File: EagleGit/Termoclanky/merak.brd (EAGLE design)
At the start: 71.1 x 39 mm, 14 parts

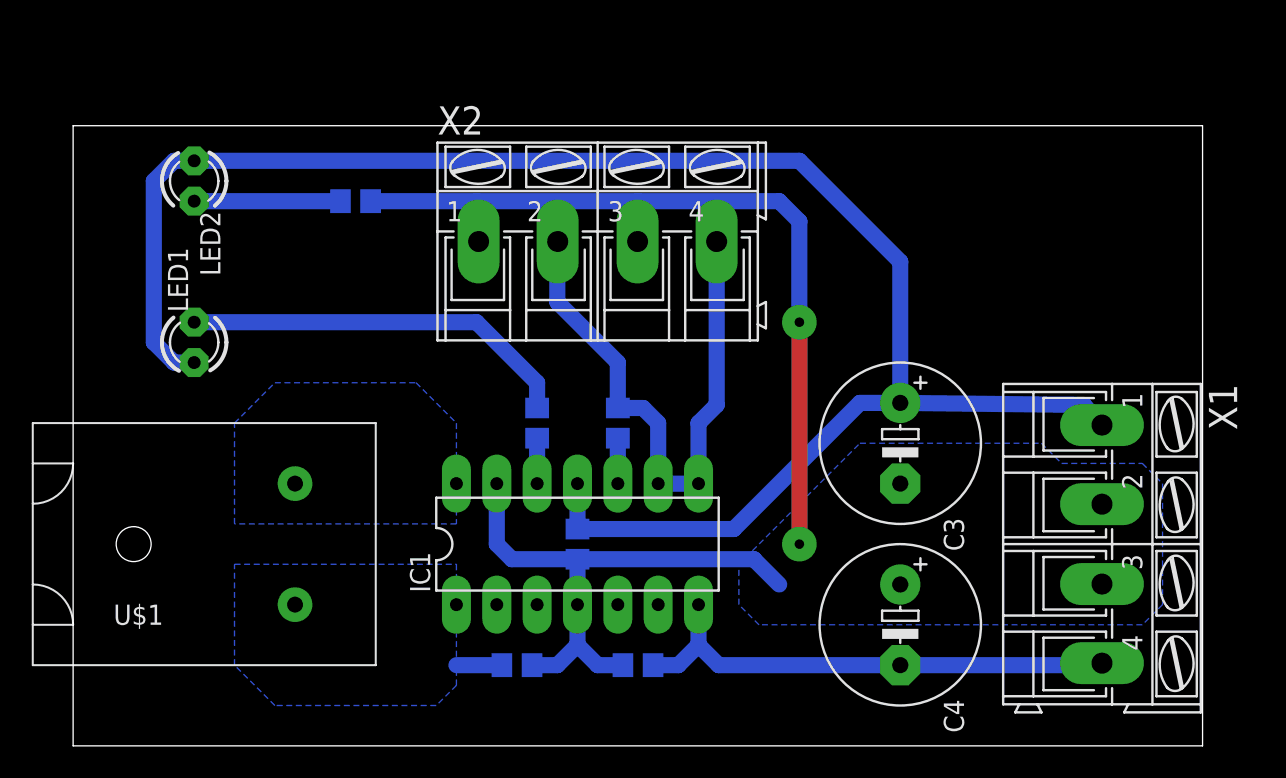
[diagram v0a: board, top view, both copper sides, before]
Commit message: Termoclanky + manuskript: - priprava do rtf
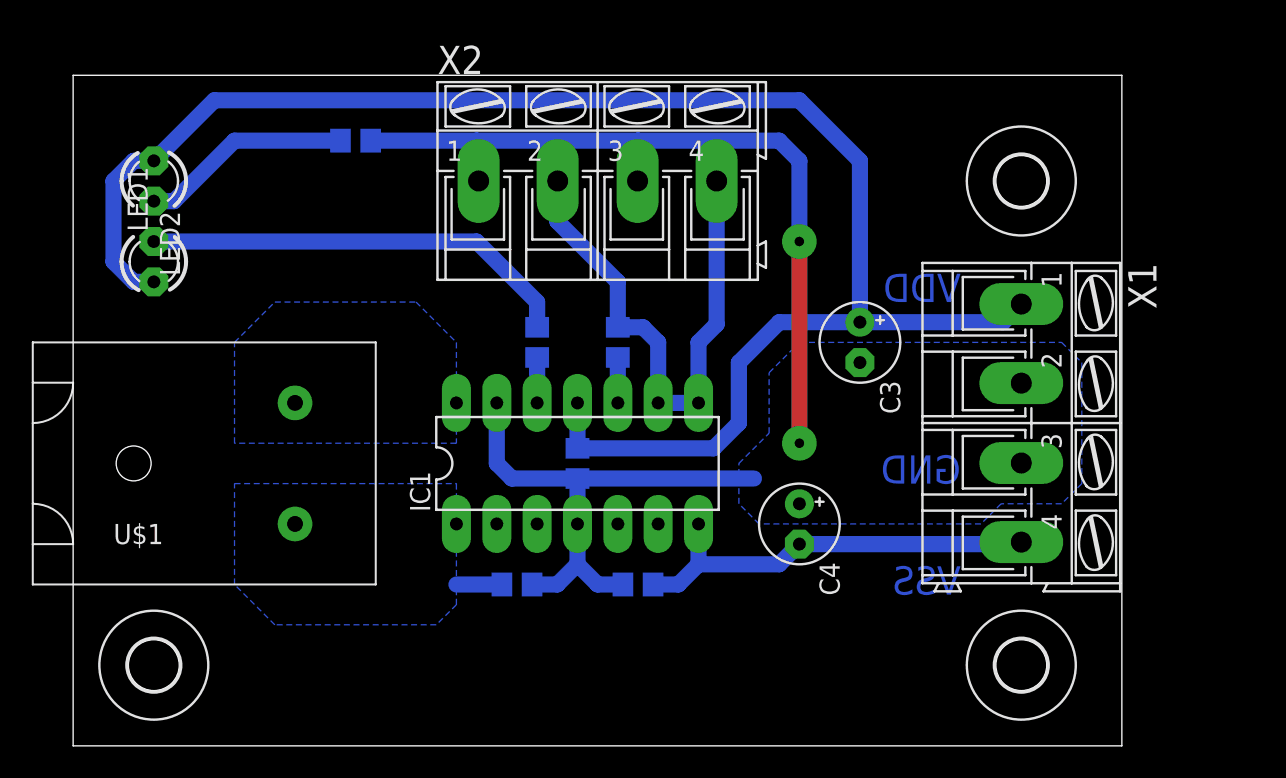
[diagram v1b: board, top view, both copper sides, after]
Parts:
- added U$2, U$3, U$4: (no value), holes:3,2
- C1, C2: value (none) -> 10n
- C3, C4: value (none) -> 10u; device rcl:E5-10,5 -> rcl:E2,5-5
- R1: value (none) -> 2k2
- moved X1 9.16 mm to (59.7, 20.3)
- moved C4 8.98 mm to (45.7, 14.0)
- moved C3 6.84 mm to (49.5, 25.4)
- moved LED1 5.68 mm to (5.08, 30.5)
- moved C1 5.08 mm to (31.8, 17.8)
- moved IC1 5.08 mm to (31.8, 17.8)
- moved U$1 5.08 mm to (11.4, 17.8)
- moved C2 5.08 mm to (35.6, 10.2)
- moved R1 5.08 mm to (27.9, 10.2)
- moved C5 5.08 mm to (34.3, 25.4)
- moved R2 5.08 mm to (29.2, 25.4)
- moved R3 3.81 mm to (17.8, 38.1)
- moved X2 3.81 mm to (33.0, 35.6)
- moved LED2 2.54 mm to (5.08, 35.6)
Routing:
- net VDD: track 112.0 -> 105.8 mm
- net VSS: track 31.9 -> 26.8 mm
- net GND: track 87.8 -> 83.0 mm
- net N$6: track 9.21 -> 13.3 mm
- net N$1: track 37.1 -> 34.5 mm
- net N$5: track 24.8 -> 27.3 mm
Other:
- board size 71.1 x 39 mm -> 66 x 42.2 mm
- board text added: "GND"
- board text added: "VDD"
- board text added: "VSS"

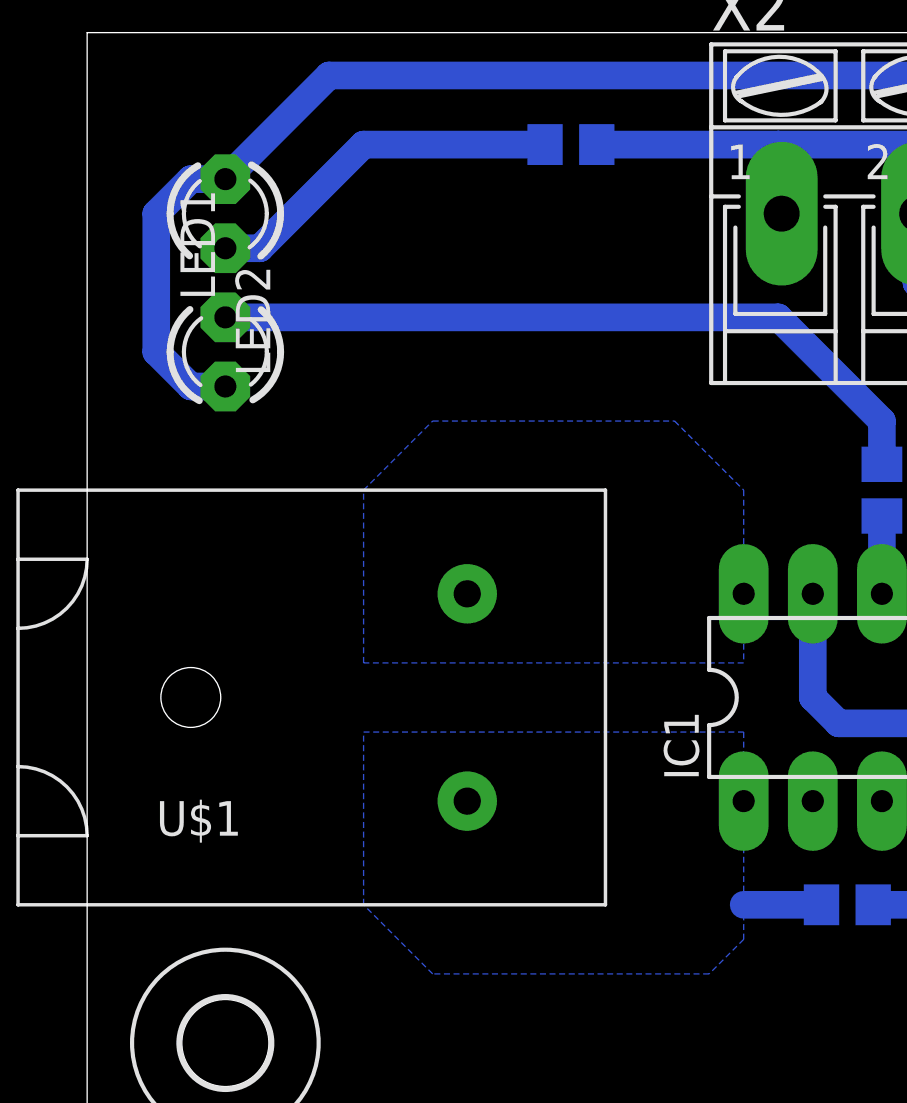
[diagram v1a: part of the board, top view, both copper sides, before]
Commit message: Eagle: - Risa zdroj - Kovanda termoclanky - Quanti akcelerometr
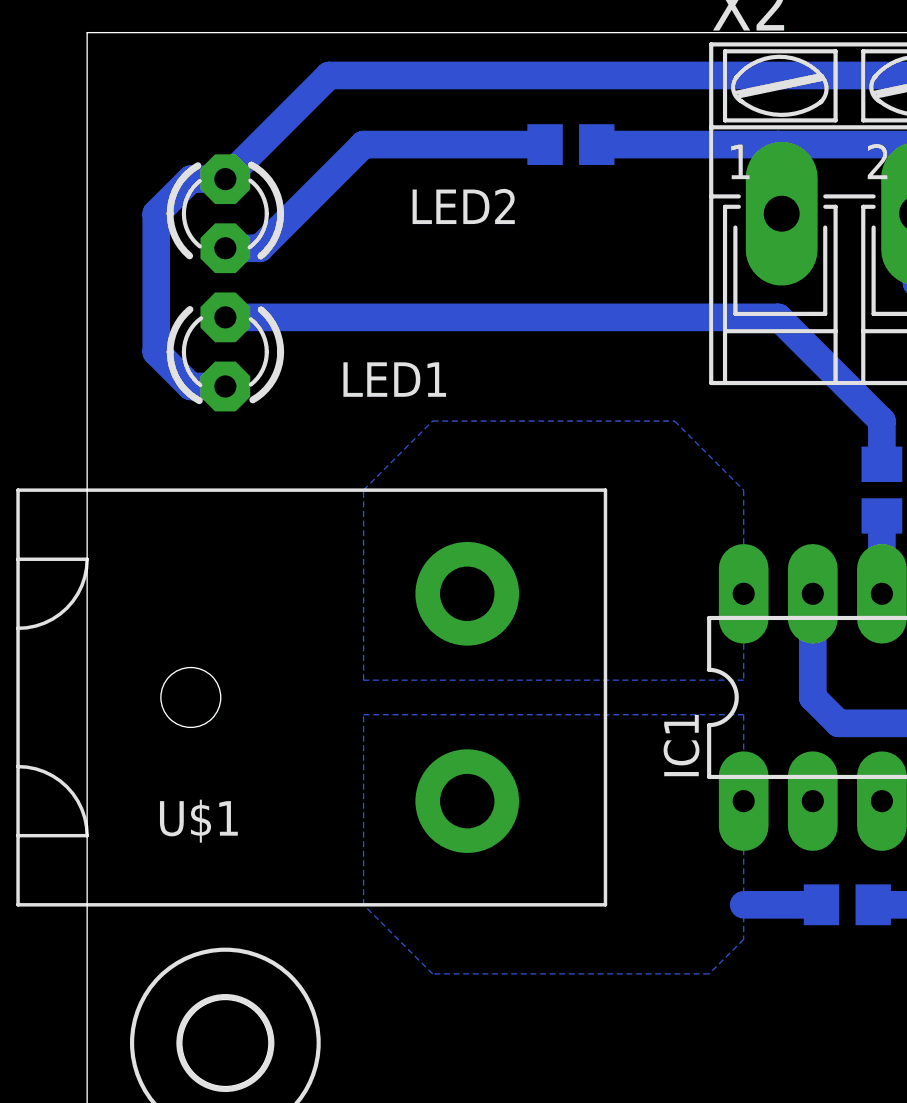
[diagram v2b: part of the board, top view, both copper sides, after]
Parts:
- LED1: value (none) -> ZLUTA
- LED2: value (none) -> CERVENA
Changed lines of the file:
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@@
 <layer number="46" name="Milling" color="3" fill="1" visible="no" active="yes"/>
 <layer number="47" name="Measures" color="7" fill="1" visible="no" active="yes"/>
-<layer number="48" name="Document" color="7" fill="1" visible="yes" active="yes"/>
-<layer number="49" name="Reference" color="7" fill="1" visible="yes" active="yes"/>
-<layer number="51" name="tDocu" color="7" fill="1" visible="yes" active="yes"/>
-<layer number="52" name="bDocu" color="7" fill="1" visible="yes" active="yes"/>
+<layer number="48" name="Document" color="7" fill="1" visible="no" active="yes"/>
+<layer number="49" name="Reference" color="7" fill="1" visible="no" active="yes"/>
+<layer number="51" name="tDocu" color="7" fill="1" visible="no" active="yes"/>
+<layer number="52" name="bDocu" color="7" fill="1" visible="no" active="yes"/>
 <layer number="90" name="Modules" color="5" fill="1" visible="no" active="no"/>
 <layer number="91" name="Nets" color="2" fill="1" visible="no" active="no"/>
@@
 <attribute name="OC_FARNELL" value="409194" x="31.75" y="17.78" size="1.778" layer="27" display="off"/>
 </element>
-<element name="LED1" library="led" package="LED3MM" value="" x="5.08" y="30.48" rot="R90"/>
-<element name="LED2" library="led" package="LED3MM" value="" x="5.08" y="35.56" rot="R270"/>
+<element name="LED1" library="led" package="LED3MM" value="ZLUTA" x="5.08" y="30.48" smashed="yes" rot="R90">
+<attribute name="NAME" x="13.335" y="30.099" size="1.27" layer="25" ratio="10" rot="R180"/>
+<attribute name="VALUE" x="13.335" y="28.321" size="1.27" layer="27" ratio="10" rot="R180"/>
+</element>
+<element name="LED2" library="led" package="LED3MM" value="CERVENA" x="5.08" y="35.56" smashed="yes" rot="R270">
+<attribute name="NAME" x="15.875" y="36.449" size="1.27" layer="25" ratio="10" rot="R180"/>
+<attribute name="VALUE" x="15.875" y="34.671" size="1.27" layer="27" ratio="10" rot="R180"/>
+</element>
 <element name="R1" library="resistor" package="R0805" value="2k2" x="27.94" y="10.16" rot="MR180"/>
 <element name="R2" library="resistor" package="R0805" value="2k2" x="29.21" y="25.4" rot="MR90"/>
@@
 <wire x1="26.99" y1="10.16" x2="24.13" y2="10.16" width="1.016" layer="16"/>
 <polygon width="0.6096" layer="16">
-<vertex x="10.16" y="16.51"/>
-<vertex x="24.13" y="16.51"/>
+<vertex x="10.16" y="17.145"/>
+<vertex x="24.13" y="17.145"/>
 <vertex x="24.13" y="8.89"/>
 <vertex x="22.86" y="7.62"/>
@@
 <contactref element="U$1" pad="MINUS"/>
 <polygon width="0.6096" layer="16">
-<vertex x="24.13" y="19.05"/>
-<vertex x="10.16" y="19.05"/>
+<vertex x="24.13" y="18.415"/>
+<vertex x="10.16" y="18.415"/>
 <vertex x="10.16" y="25.4"/>
 <vertex x="12.7" y="27.94"/>
